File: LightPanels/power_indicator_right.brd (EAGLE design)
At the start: 47.5 x 48 mm, 22 parts

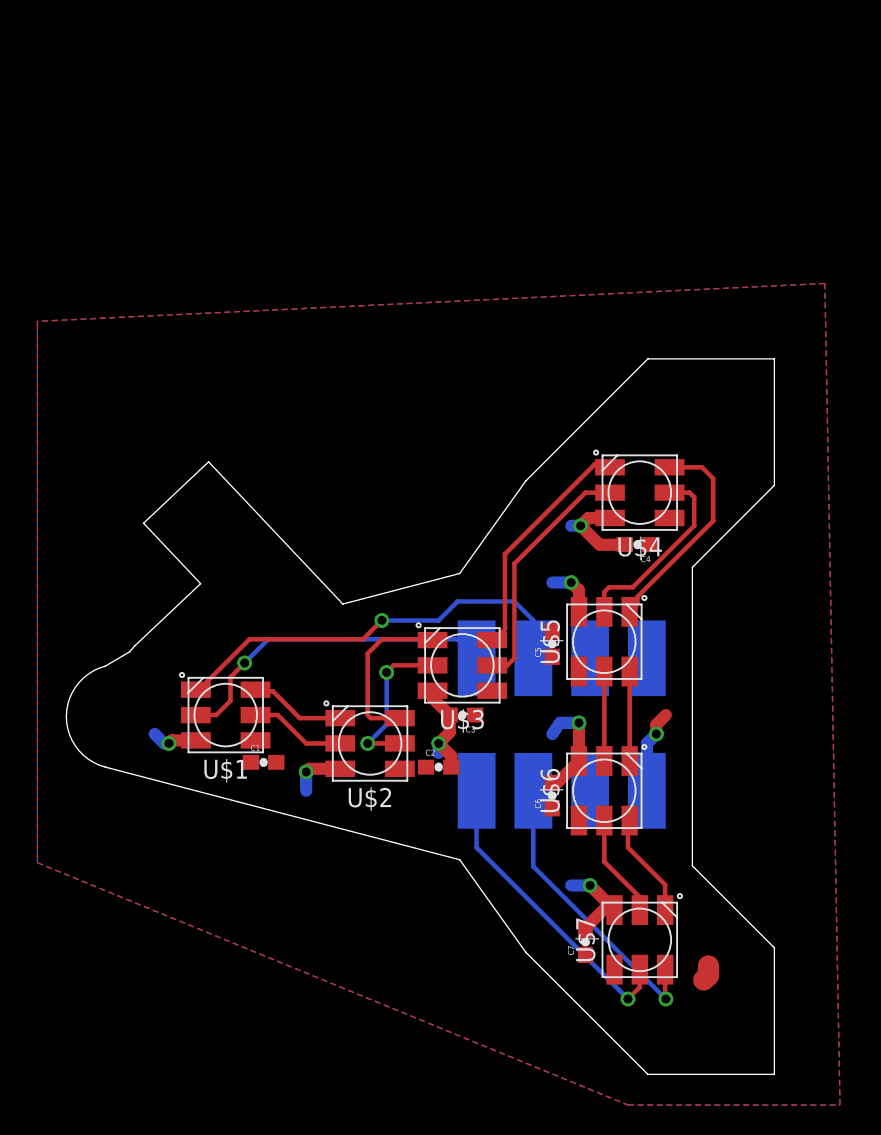
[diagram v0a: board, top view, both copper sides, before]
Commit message: Latest light panel pcb files
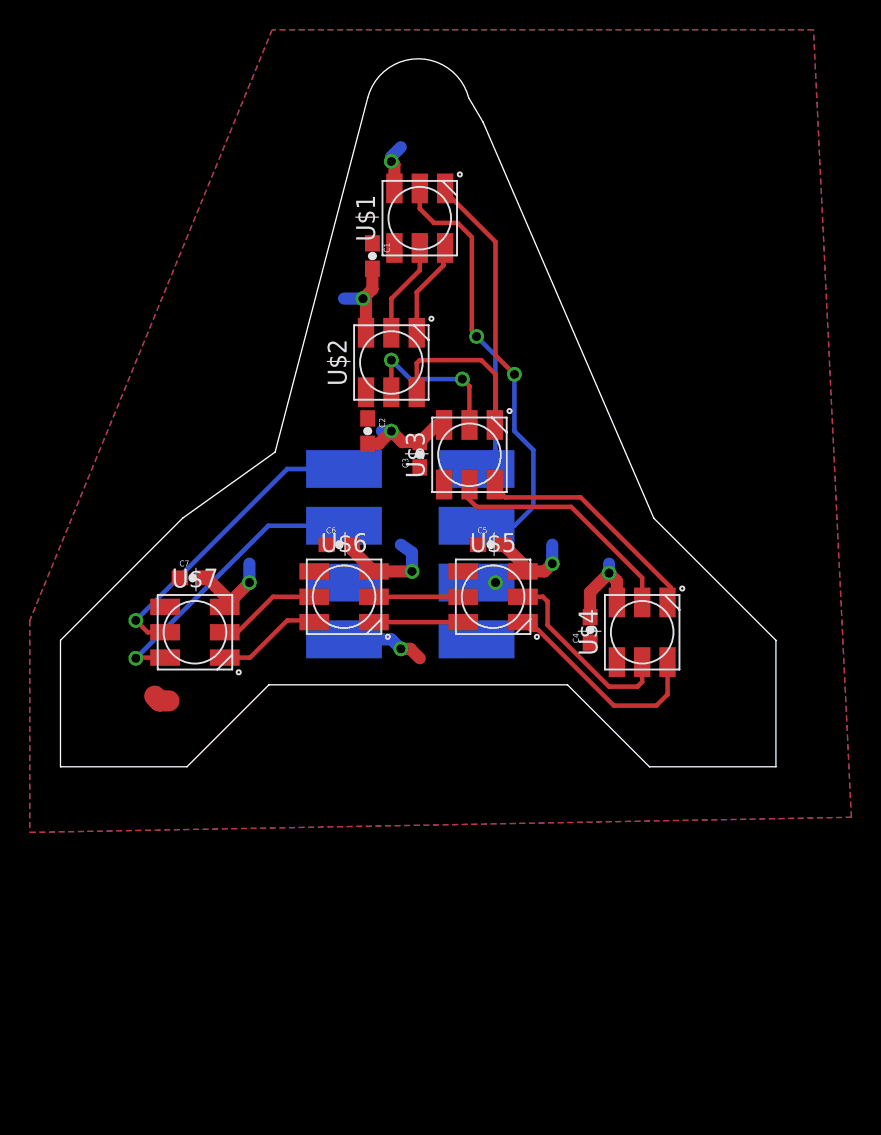
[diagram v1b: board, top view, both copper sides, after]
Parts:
- moved U$7 36.3 mm to (9.05, 9.37), turned to 180 degrees
- moved C7 35.9 mm to (8.89, 13.0), turned to 0 degrees
- moved U$1 35.8 mm to (24.1, 37.1), turned to 270 degrees
- moved C1 34.7 mm to (21.0, 34.6), turned to 270 degrees
- moved U$2 25.6 mm to (22.2, 27.5), turned to 270 degrees
- moved PAD8 23.3 mm to (19.1, 20.3), turned to 90 degrees
- moved C2 23.0 mm to (20.6, 22.9), turned to 270 degrees
- moved PAD6 22.7 mm to (19.1, 8.89), turned to 90 degrees
- moved C6 22.1 mm to (18.7, 15.2), turned to 0 degrees
- moved PAD7 21.8 mm to (19.1, 16.5), turned to 90 degrees
- moved U$6 21.8 mm to (19.1, 11.7), turned to 180 degrees
- moved PAD5 21.6 mm to (19.1, 12.7), turned to 90 degrees
- moved C3 17.7 mm to (24.1, 21.3), turned to 90 degrees
- moved U$3 14.1 mm to (27.5, 21.3), turned to 270 degrees
- moved PAD4 12.7 mm to (27.9, 20.3), turned to 90 degrees
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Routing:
- net GND: track 36.5 -> 41.1 mm
- net +5V: track 6.69 -> 7.96 mm, vias 1 -> 2
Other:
- board size 47.5 x 48 mm -> 48 x 47.5 mm
